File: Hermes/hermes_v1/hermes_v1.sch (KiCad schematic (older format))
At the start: 13 parts, among them IC1 LD39200PU33R, P1 5V_BAT, P2 GND_BAT

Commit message: routed rp2040
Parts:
- IC1: symbol LD39200PU33R:LD39200PU33R -> hermes_v1-rescue:LD39200PU33R-LD39200PU33R
- P1, P2: symbol pkl_misc:PAD_SMD -> hermes_v1-rescue:PAD_SMD-pkl_misc
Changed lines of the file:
@@
 $EndSheet
 $Comp
-L LD39200PU33R:LD39200PU33R IC1
+L hermes_v1-rescue:LD39200PU33R-LD39200PU33R IC1
 U 1 1 60E8DF86
 P 8400 5100
@@
 $EndComp
 $Comp
-L pkl_misc:PAD_SMD P1
+L hermes_v1-rescue:PAD_SMD-pkl_misc P1
 U 1 1 61092F85
 P 1150 1950
@@
 $EndComp
 $Comp
-L pkl_misc:PAD_SMD P2
+L hermes_v1-rescue:PAD_SMD-pkl_misc P2
 U 1 1 6109405B
 P 1150 2150

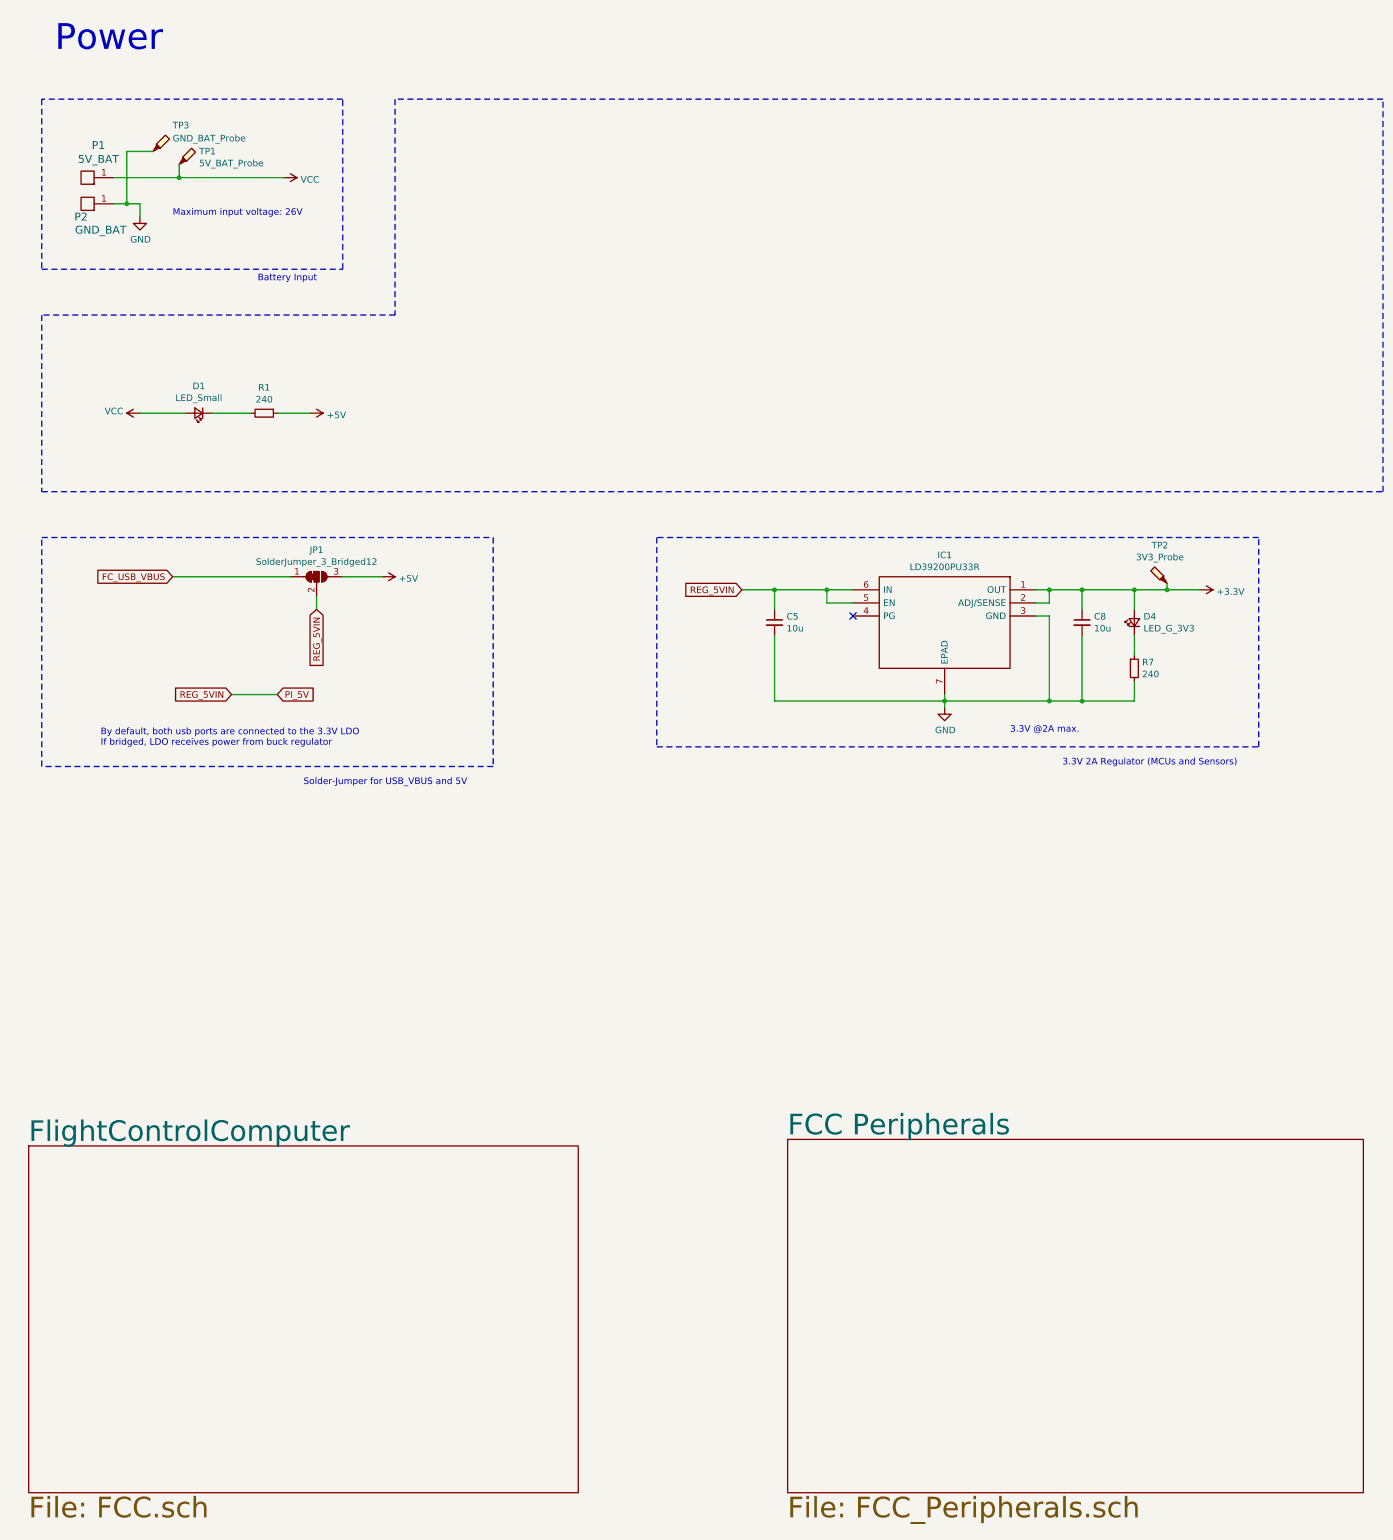
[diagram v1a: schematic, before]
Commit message: new
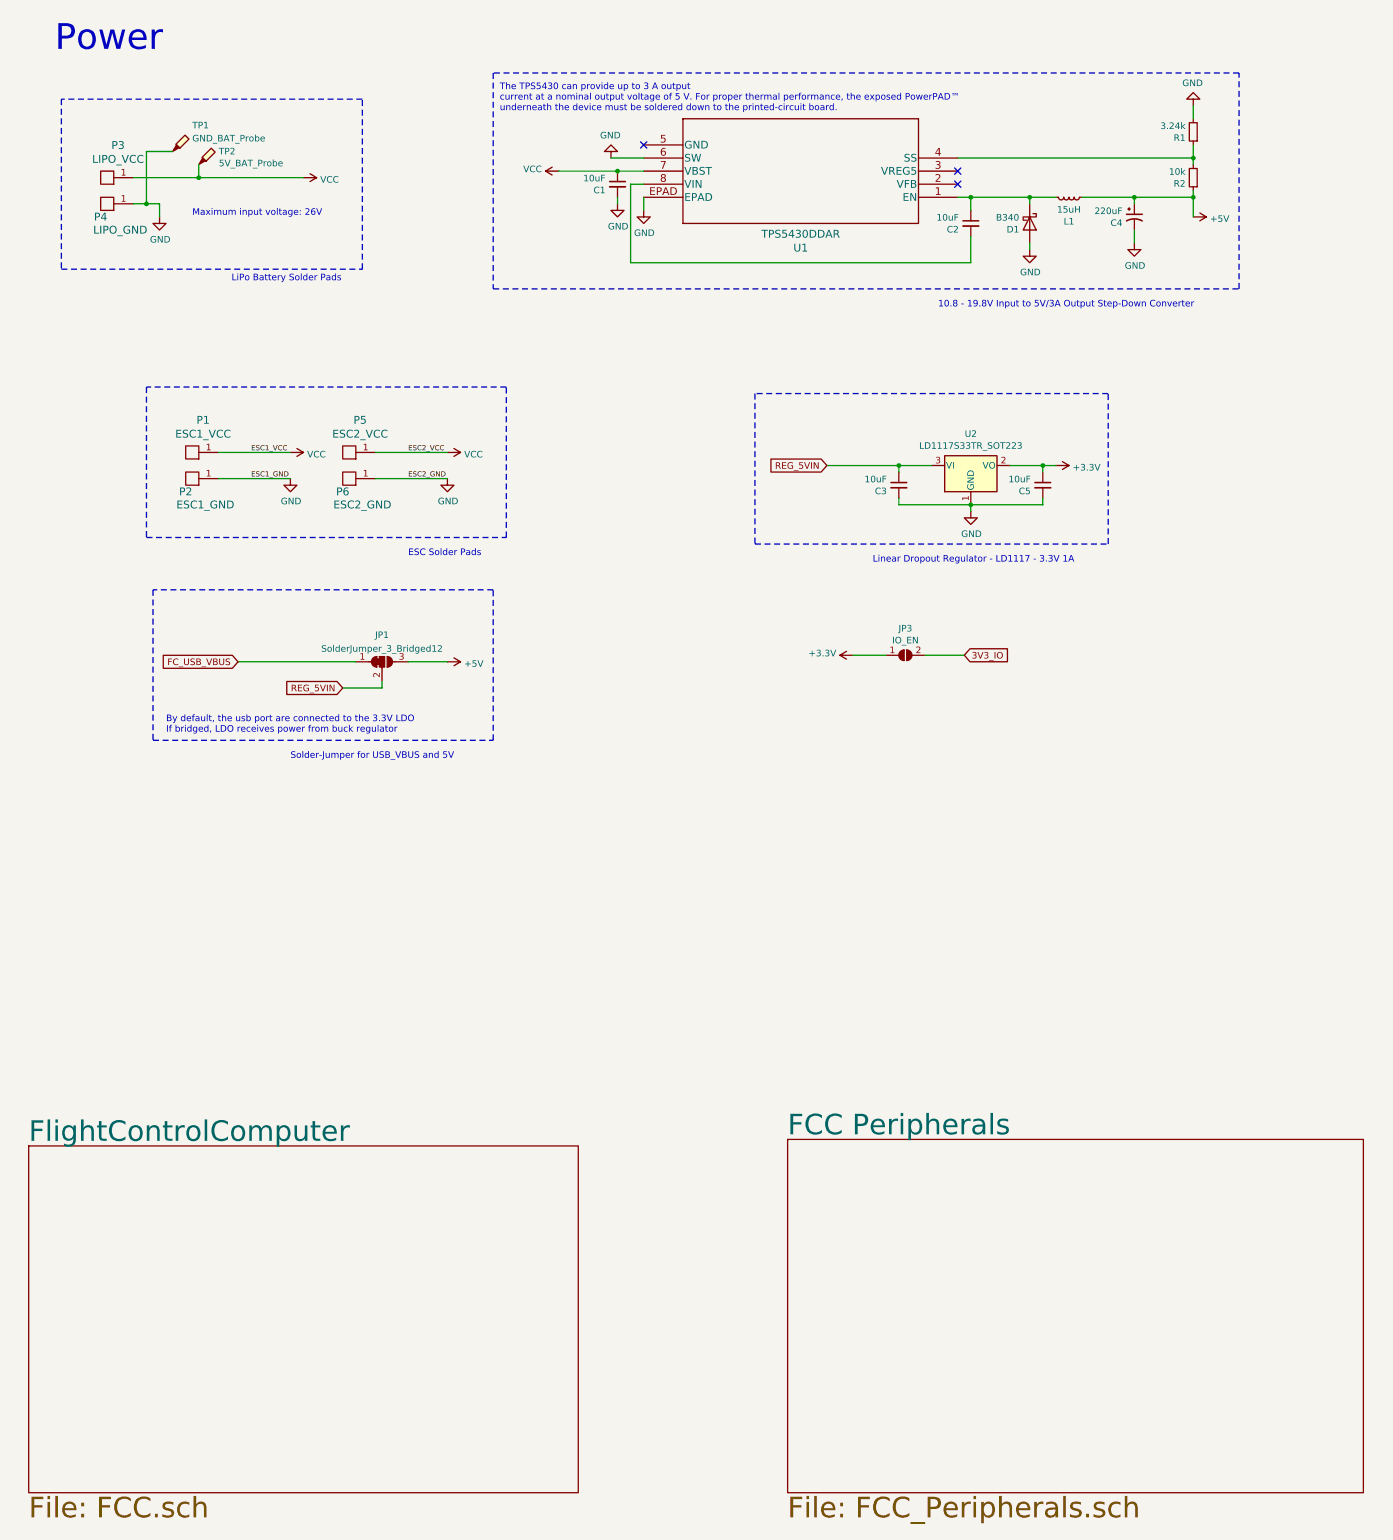
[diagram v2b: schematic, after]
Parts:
- removed C8: 10u, Capacitor_SMD:C_0402_1005Metric_Pad0.74x0.62mm_HandSolder, symbol Device:C_Small
- removed D1: LED_Small, LED_SMD:LED_0402_1005Metric_Pad0.77x0.64mm_HandSolder, symbol Device:LED_Small
- removed D4: LED_G_3V3, LED_SMD:LED_0402_1005Metric_Pad0.77x0.64mm_HandSolder, symbol Device:LED_Small
- removed IC1: LD39200PU33R, lib:SON95P300X300X100-7N-D, symbol hermes_v1-rescue:LD39200PU33R-LD39200PU33R
- removed R7: 240, Resistor_SMD:R_0402_1005Metric_Pad0.72x0.64mm_HandSolder, symbol Device:R_Small
- removed TP2: 3V3_Probe, TestPoint:TestPoint_Pad_D1.5mm, symbol Connector:TestPoint_Probe
- added C1, C2, C3: 10uF, Capacitor_SMD:C_0402_1005Metric_Pad0.74x0.62mm_HandSolder, symbol Device:C_Small
- added C4: 220uF, Capacitor_SMD:CP_Elec_6.3x5.4, symbol Device:CP1_Small
- added D1: B340, Diode_SMD:D_SMC, symbol Diode:B340
- added JP3: IO_EN, Jumper:SolderJumper-2_P1.3mm_Open_RoundedPad1.0x1.5mm, symbol Jumper:SolderJumper_2_Open
- added L1: 15uH, Inductor_SMD:L_0402_1005Metric, symbol Device:L_Small
- added P1: ESC1_VCC, TestPoint:TestPoint_Pad_2.0x2.0mm, symbol hermes_v1-rescue:PAD_SMD-pkl_misc
- added P2: ESC1_GND, TestPoint:TestPoint_Pad_D2.0mm, symbol hermes_v1-rescue:PAD_SMD-pkl_misc
- added P5: ESC2_VCC, TestPoint:TestPoint_Pad_2.0x2.0mm, symbol hermes_v1-rescue:PAD_SMD-pkl_misc
- added P6: ESC2_GND, TestPoint:TestPoint_Pad_D2.0mm, symbol hermes_v1-rescue:PAD_SMD-pkl_misc
- added R2: 10k, Resistor_SMD:R_0402_1005Metric_Pad0.72x0.64mm_HandSolder, symbol Device:R_Small
- added U1: TPS5430DDAR, TPS5430DDAR:TPS5430DDAR, symbol TPS5430DDAR:TPS5430DDAR
- added U2: LD1117S33TR_SOT223, Package_TO_SOT_SMD:SOT-223-3_TabPin2, symbol Regulator_Linear:LD1117S33TR_SOT223
- C5: value 10u -> 10uF
- P3: renamed from P1; value 5V_BAT -> LIPO_VCC
- P4: renamed from P2; value GND_BAT -> LIPO_GND
- R1: value 240 -> 3.24k
- TP1: renamed from TP3; footprint TestPoint:TestPoint_Pad_D1.5mm -> TestPoint:TestPoint_Pad_D1.0mm
- TP2: renamed from TP1; footprint TestPoint:TestPoint_Pad_D1.5mm -> TestPoint:TestPoint_Pad_D1.0mm
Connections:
- net +3V3: now also C5.1, JP3.1 (A), U2.2 (VO)
- net +5V: now also C4.1, L1.1, R2.1; no longer R1.1
- net GND: now also R1.2, C1.2, C3.2, C4.2, D1.2 (A), P2.1 (PAD), P6.1 (PAD), U1.6 (SW), U1.EPAD, U2.1 (GND)
- net VCC: now also C1.1, P1.1 (PAD), P5.1 (PAD), U1.7 (VBST)
- net PI_5V renamed REG_5VIN
- net REG_5VIN: now also C3.1, U2.3 (VI); no longer C5.1
- new net: C2.1, D1.1 (K), L1.2, U1.1 (EN)
- new net: R1.1, R2.2, U1.4 (SS)
- new net: C2.2, U1.8 (VIN)
- new net 3V3_IO: JP3.2 (B)
- no-connect marks 1 -> 3
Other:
- note added: "10.8 - 19.8V Input to 5V/3A Output Step-Down Converter"
- note added: "By default, the usb port are connected to the 3.3V LDO\nIf bridged, LDO receives power from buck regulator"
- note added: "ESC Solder Pads"
- note added: "LiPo Battery Solder Pads"
- note added: "Linear Dropout Regulator - LD1117 - 3.3V 1A"
- note added: "The TPS5430 can provide up to 3 A output\ncurrent at a nominal output voltage of 5 V. For proper thermal performance, the exposed PowerPAD™\nunderneath the device must be soldered down to the printed-circuit board."
- note removed: "3.3V 2A Regulator (MCUs and Sensors)"
- note removed: "3.3V @2A max."
- note removed: "Battery Input"
- note removed: "By default, both usb ports are connected to the 3.3V LDO\nIf bridged, LDO receives power from buck regulator"
- moved on the sheet: JP1, P3, P4, TP1, TP2
